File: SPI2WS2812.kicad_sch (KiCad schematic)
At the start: 17 parts, among them J3 Conn_01x06, T1 2N7002, T2 2N7002, T3 2N7002, T4 BSS84

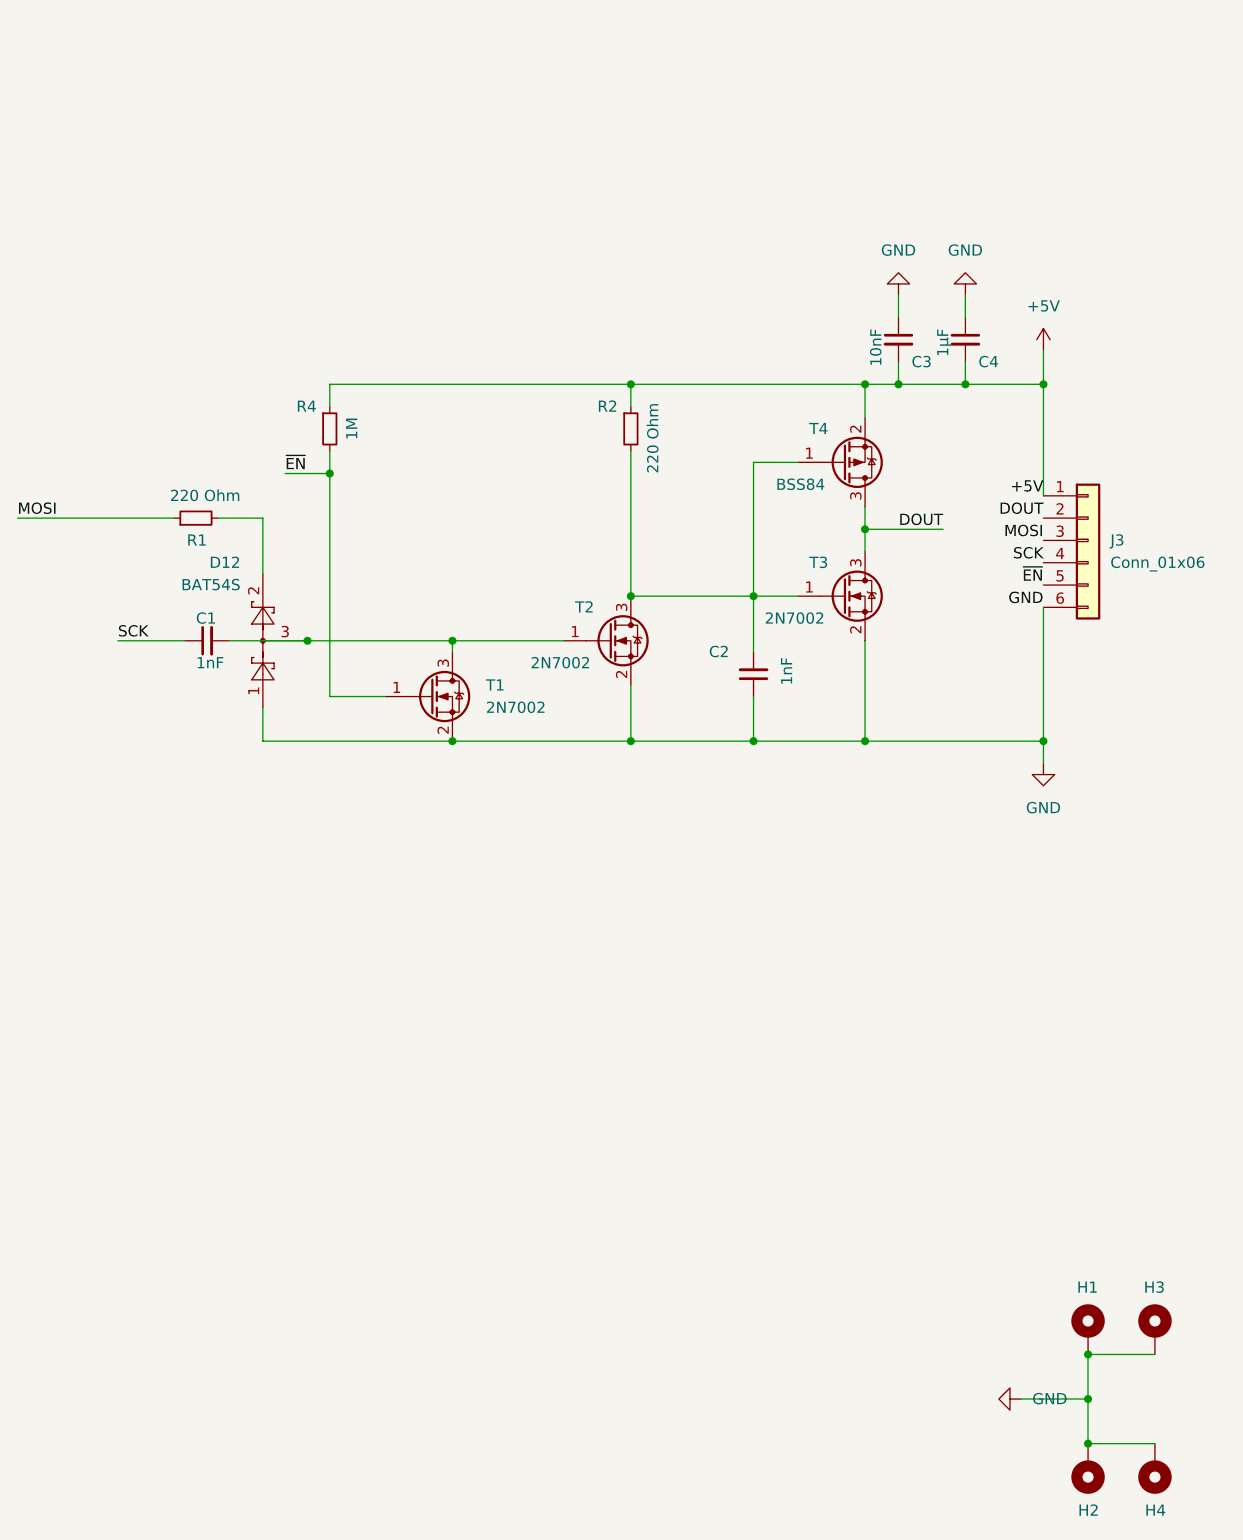
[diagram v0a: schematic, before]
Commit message: git-svn-id: file:///D/00%20-%20Dev%20&%20Calculs/RepoTortoiseSVN_PCB/SPI2WS2812/trunk@13 14acadc8-6264-6a46-bd6b-d9c895d7e7fb
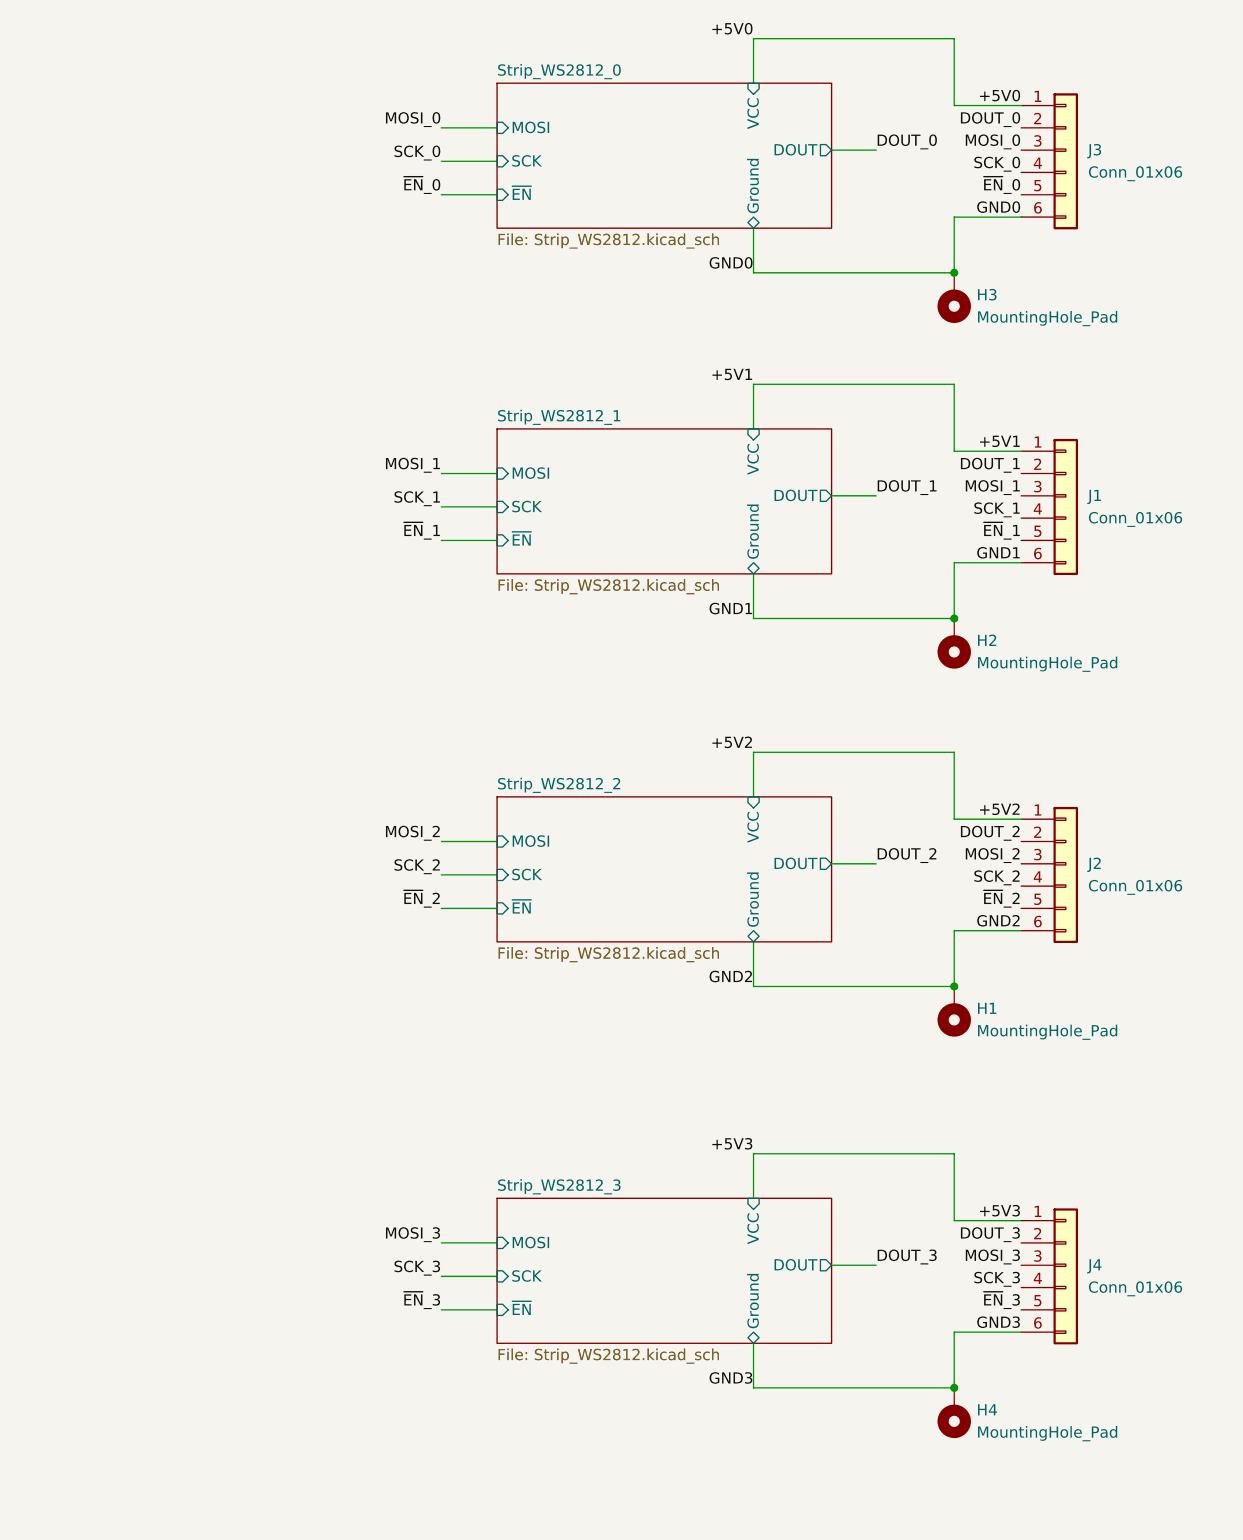
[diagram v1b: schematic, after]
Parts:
- removed C1, C2: 1nF, Capacitor_SMD:C_1210_3225Metric_Pad1.33x2.70mm_HandSolder, symbol Device:C_Small
- removed C3: 10nF, Capacitor_SMD:C_1210_3225Metric_Pad1.33x2.70mm_HandSolder, symbol Device:C_Small
- removed C4: 1µF, Capacitor_SMD:C_1210_3225Metric_Pad1.33x2.70mm_HandSolder, symbol Device:C_Small
- removed D12: BAT54S, Package_TO_SOT_SMD:SOT-23, symbol Diode:BAT54S
- removed R1, R2: 220 Ohm, Resistor_SMD:R_1210_3225Metric_Pad1.30x2.65mm_HandSolder, symbol Device:R_Small
- removed R4: 1M, Resistor_SMD:R_1210_3225Metric_Pad1.30x2.65mm_HandSolder, symbol Device:R_Small
- removed T1, T2, T3: 2N7002, Package_TO_SOT_SMD:SOT-23_Handsoldering, symbol Transistor_FET:2N7002
- removed T4: BSS84, Package_TO_SOT_SMD:SOT-23_Handsoldering, symbol Transistor_FET:BSS84
- added J1, J2, J4: Conn_01x06, Connector_PinHeader_2.54mm:PinHeader_1x06_P2.54mm_Vertical, symbol Connector_Generic:Conn_01x06
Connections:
- net +5V renamed +5V0
- net DOUT renamed DOUT_0
- removed net GND: H1.1, H2.1, H3.1, H4.1, J3.6 (Pin_6)
- net MOSI renamed MOSI_0
- net SCK renamed SCK_0
- net ~{EN} renamed ~{EN}_0
- new net +5V1: J1.1 (Pin_1)
- new net +5V2: J2.1 (Pin_1)
- new net +5V3: J4.1 (Pin_1)
- new net DOUT_1: J1.2 (Pin_2)
- new net DOUT_2: J2.2 (Pin_2)
- new net DOUT_3: J4.2 (Pin_2)
- new net GND0: H3.1, J3.6 (Pin_6)
- new net GND1: H2.1, J1.6 (Pin_6)
- new net GND2: H1.1, J2.6 (Pin_6)
- new net GND3: H4.1, J4.6 (Pin_6)
- new net MOSI_1: J1.3 (Pin_3)
- new net MOSI_2: J2.3 (Pin_3)
- new net MOSI_3: J4.3 (Pin_3)
- new net SCK_1: J1.4 (Pin_4)
- new net SCK_2: J2.4 (Pin_4)
- new net SCK_3: J4.4 (Pin_4)
- new net ~{EN}_1: J1.5 (Pin_5)
- new net ~{EN}_2: J2.5 (Pin_5)
- new net ~{EN}_3: J4.5 (Pin_5)
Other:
- added sheet Strip_WS2812_0 (Strip_WS2812.kicad_sch)
- added sheet Strip_WS2812_1 (Strip_WS2812.kicad_sch)
- added sheet Strip_WS2812_2 (Strip_WS2812.kicad_sch)
- added sheet Strip_WS2812_3 (Strip_WS2812.kicad_sch)
- moved on the sheet: J3
